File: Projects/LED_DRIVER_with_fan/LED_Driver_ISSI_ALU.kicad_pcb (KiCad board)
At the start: 2 copper layers, 117.7 x 117.7 mm, 114 parts, among them J1 5055780871, J2 505578-0271, U1 IS31LT3360, U2 IS31LT3360, U3 IS31LT3360, U4 IS31LT3360, U5 IS31LT3360, U6 IS31LT3360

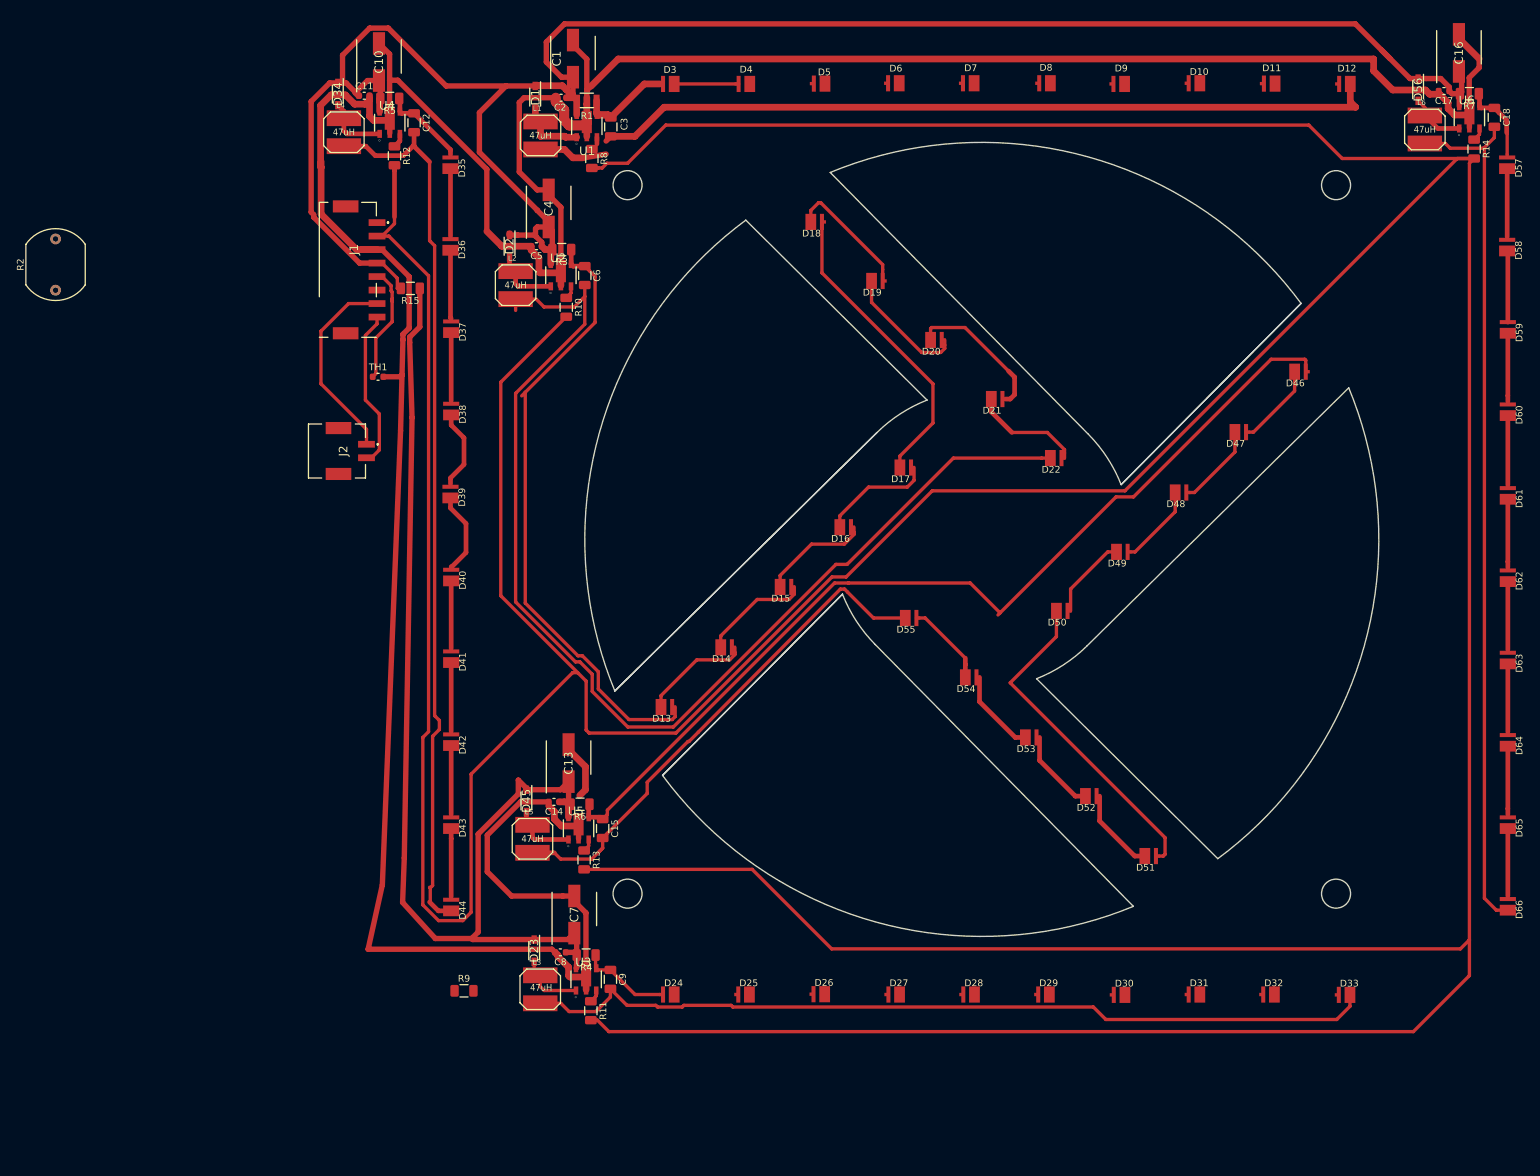
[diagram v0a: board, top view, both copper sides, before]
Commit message: added pca96...
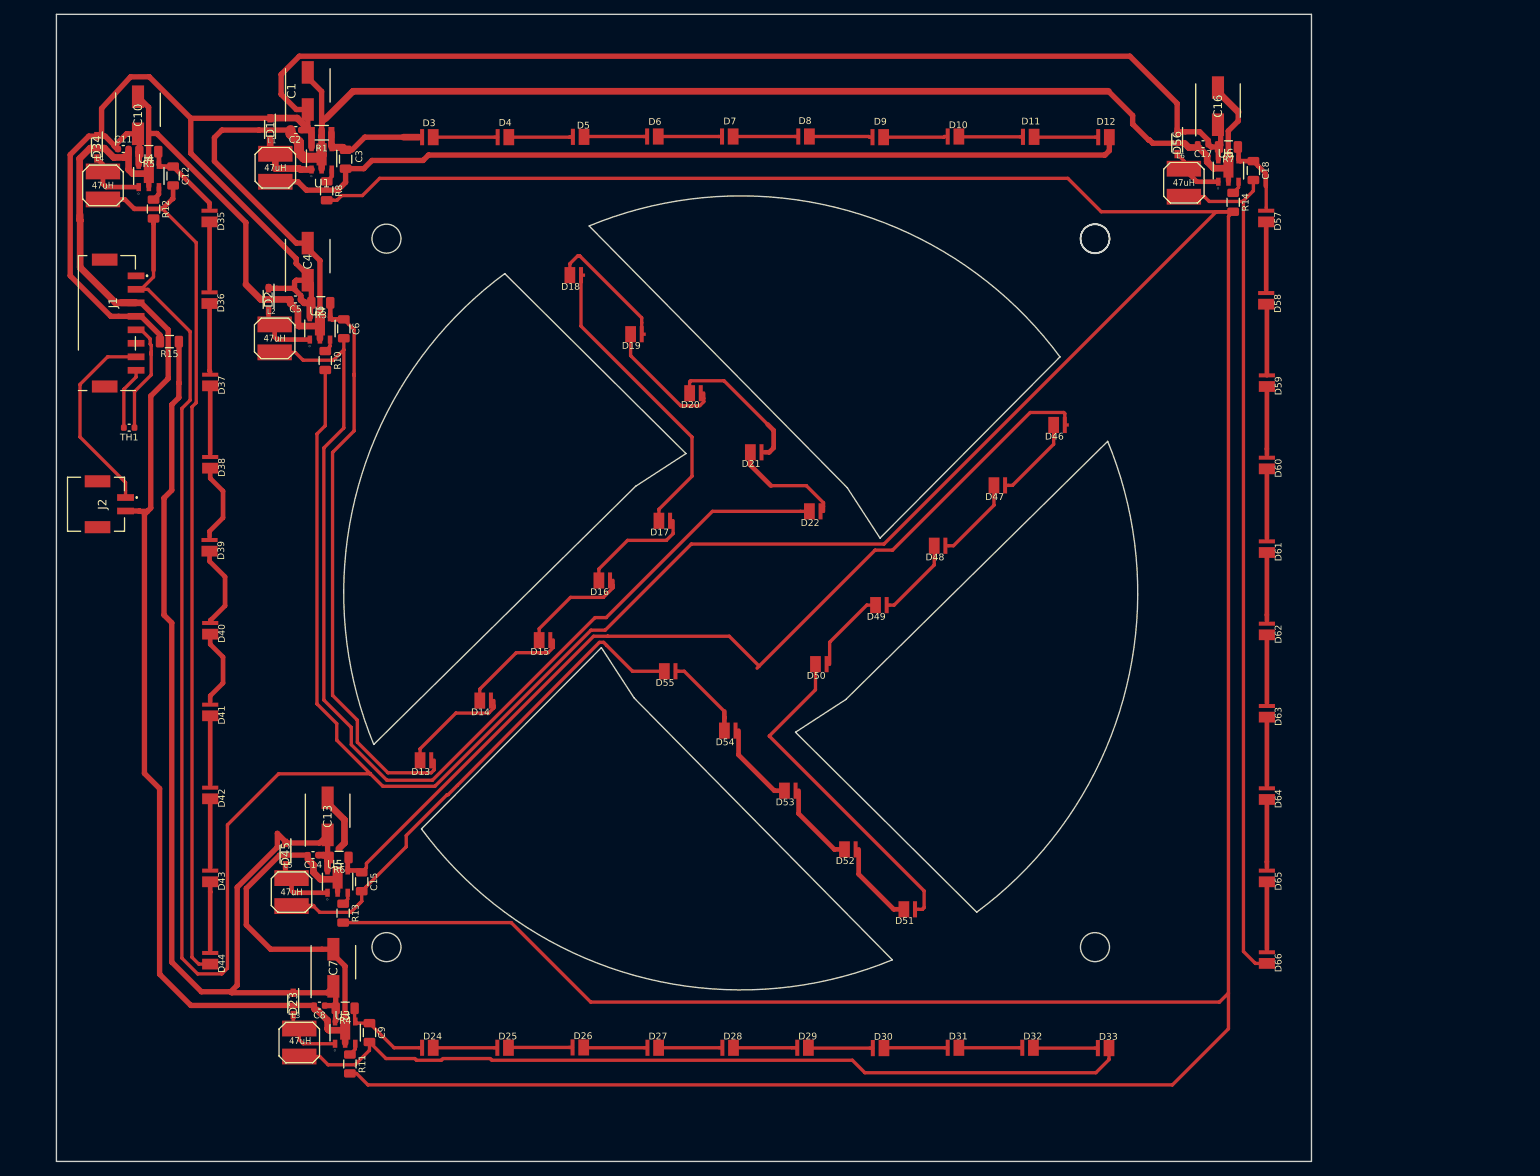
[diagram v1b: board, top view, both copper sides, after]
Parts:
- removed R2: LDR03, OptoDevice:R_LDR_10x8.5mm_P7.6mm_Vertical
- removed R9: 100, Resistor_SMD:R_1206_3216Metric
- moved C2 39.6 mm to (70.0, 31.8)
- moved C3 39.6 mm to (77.4, 36.1)
- moved L1 39.6 mm to (66.9, 37.4)
- moved C1 39.6 mm to (71.8, 26.0)
- moved D1 39.6 mm to (66.2, 31.7)
- moved R1 39.6 mm to (73.8, 32.2)
- moved R8 39.6 mm to (74.5, 40.8)
- moved U1 39.6 mm to (73.8, 36.0)
- moved TH1 37.6 mm to (45.3, 75.9), turned to 180 degrees
- moved C13 36.6 mm to (74.7, 133.5)
- moved D12 36.6 mm to (190.5, 32.8)
- moved D20 36.6 mm to (128.3, 70.8)
- moved D30 36.6 mm to (157.1, 167.8)
- moved D45 36.6 mm to (68.4, 139.1)
- moved D51 36.6 mm to (160.1, 147.3)
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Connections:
- net Net-(J1-Pad5) renamed /NTC
- net Net-(J1-Pad7) renamed /12V_Fan
- J1 pad 8: Net-(J1-Pad8) -> /3.3V
- J2 pad 2: Net-(J1-Pad8) -> GND
- TH1 pad 2: GND -> /3.3V
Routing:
- net Net-(J1-Pad8): track 23.6 -> 0.00 mm
- net GND: track 524.8 -> 537.8 mm
- net Net-(D7-Pad1): track 0.00 -> 9.65 mm
- net Net-(D32-Pad1): track 0.00 -> 9.57 mm
- net Net-(D29-Pad1): track 0.00 -> 9.57 mm
- net Net-(D10-Pad1): track 0.00 -> 9.52 mm
- net Net-(D11-Pad1): track 0.00 -> 9.52 mm
- net Net-(D25-Pad1): track 0.00 -> 9.52 mm
- net Net-(D24-Pad1): track 0.00 -> 9.50 mm
- net Net-(D30-Pad1): track 0.00 -> 9.47 mm
- net Net-(D26-Pad1): track 0.00 -> 9.47 mm
- net Net-(D27-Pad1): track 0.00 -> 9.45 mm
- net Net-(D28-Pad1): track 0.00 -> 9.45 mm
- net Net-(D31-Pad1): track 0.00 -> 9.40 mm
- net Net-(D5-Pad1): track 0.00 -> 9.37 mm
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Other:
- board size 117.7 x 117.7 mm -> 186 x 170 mm
- net class Default: clearance 0.4 -> 0.2
- rule trace_clearance: 0.4 -> 0.2

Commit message: updates to Control board and LED light
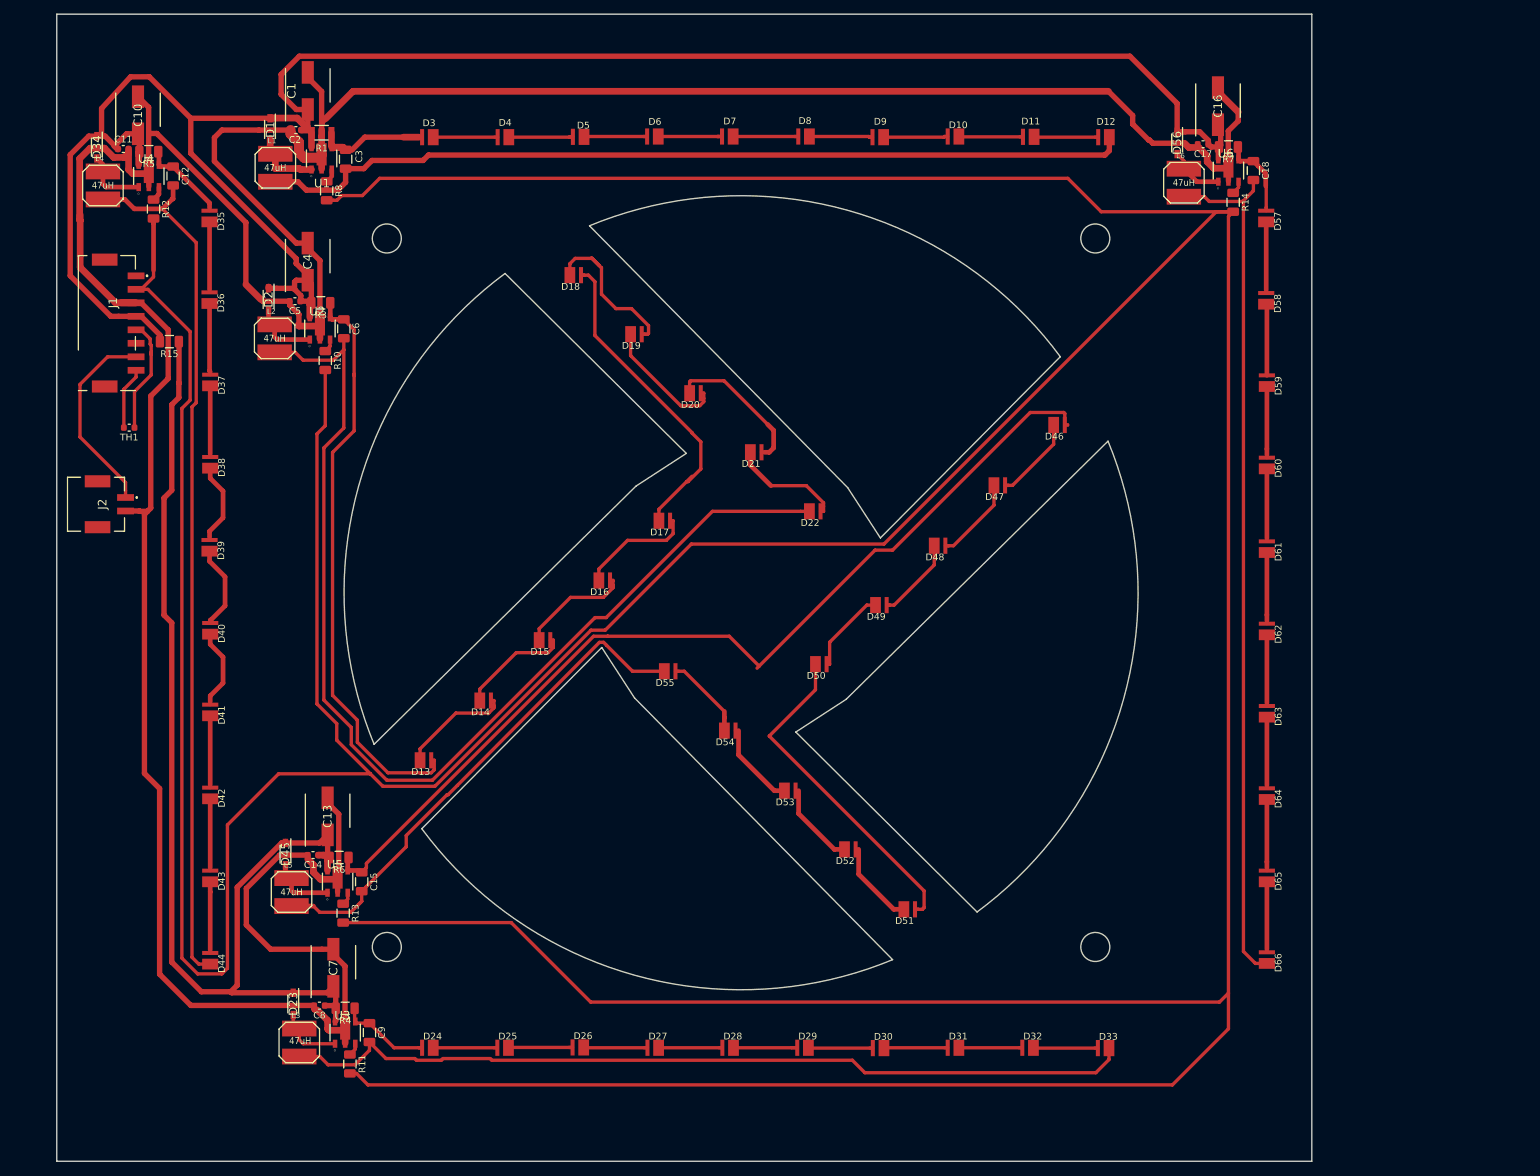
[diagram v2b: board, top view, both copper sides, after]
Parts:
- moved C5 0.27 mm to (69.8, 57.1)
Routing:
- net Net-(D18-Pad1): track 19.0 -> 23.9 mm
- net GND: track 537.8 -> 541.5 mm
- net Net-(D17-Pad1): track 45.2 -> 48.2 mm
- net VCC: track 479.1 -> 476.6 mm
- net Net-(D6-Pad1): track 9.00 -> 9.70 mm
